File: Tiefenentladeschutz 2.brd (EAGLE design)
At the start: 60 x 60 mm, 23 parts, among them IC1 ICL7665CSA, Q1 NMOSFET-D2PAK-7

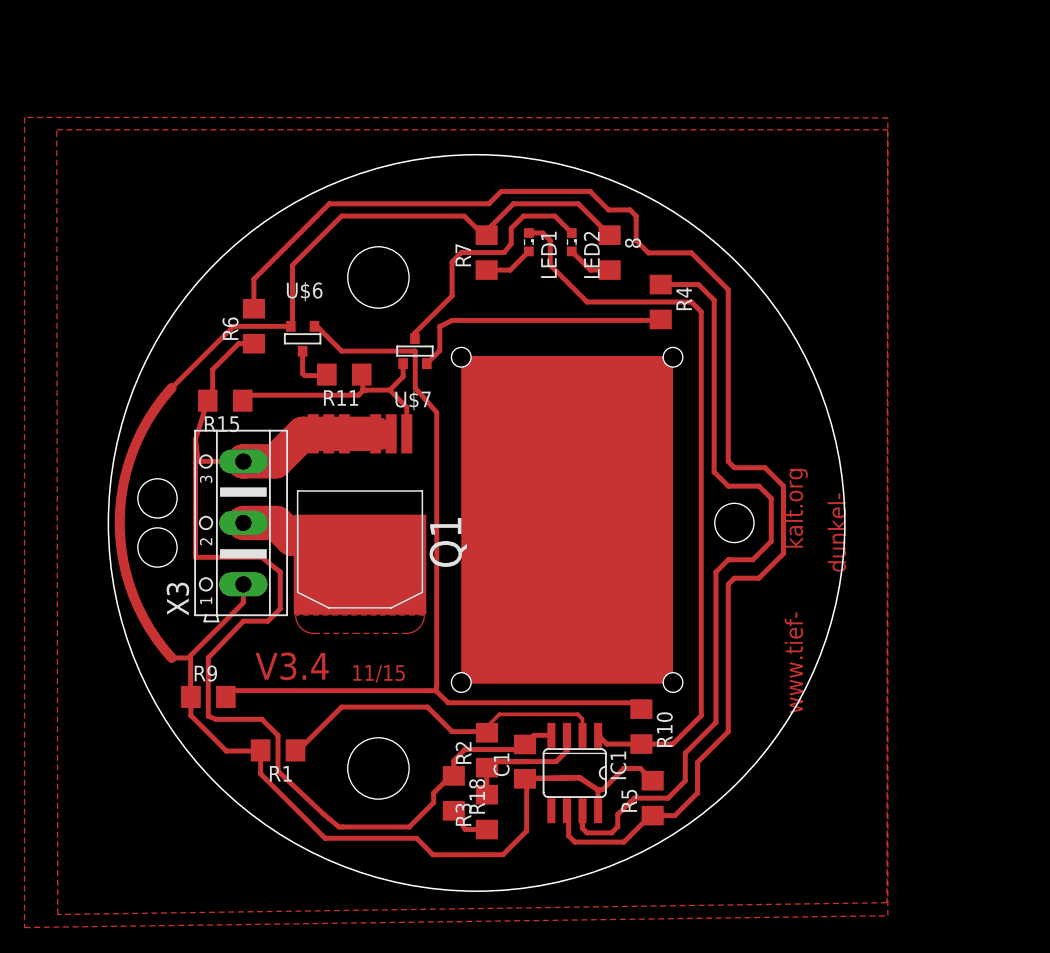
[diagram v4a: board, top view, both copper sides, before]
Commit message: 3.5
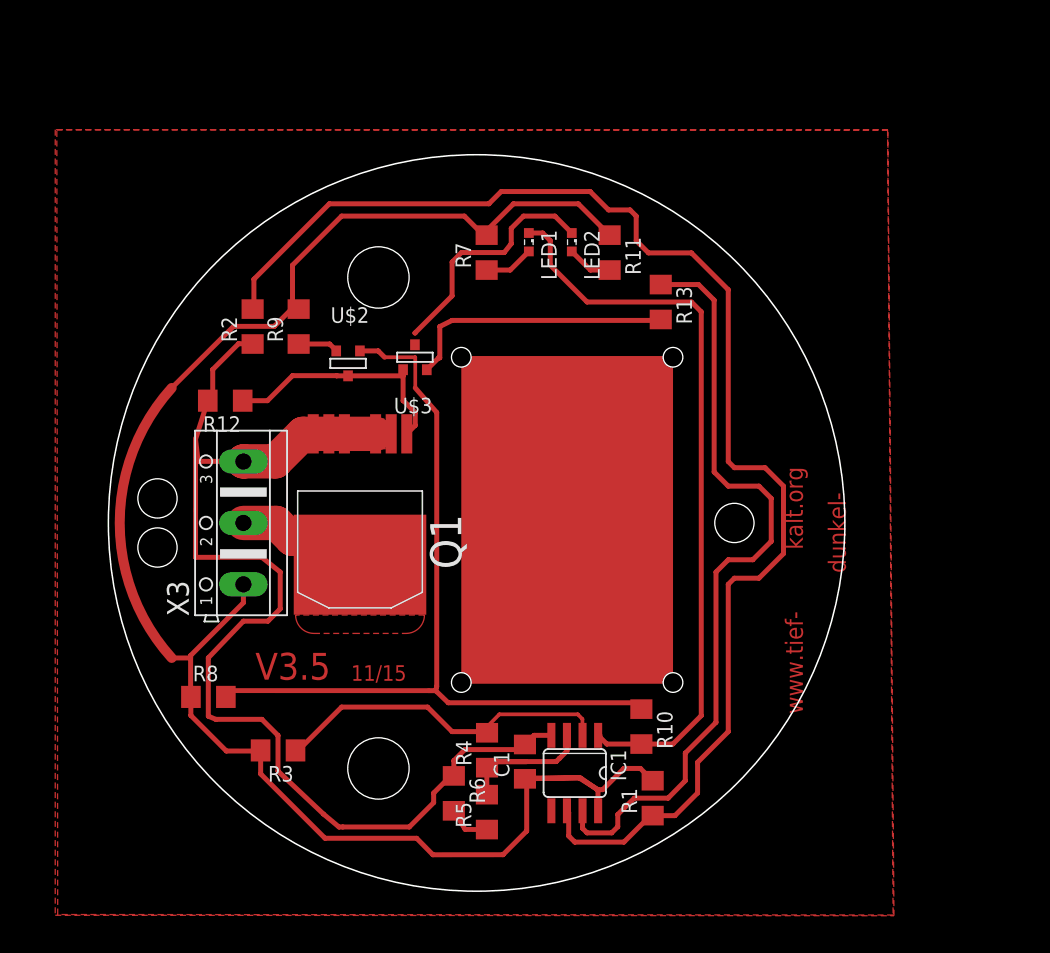
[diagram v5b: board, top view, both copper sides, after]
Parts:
- removed 8, R18: 5,6k, eagle-ltspice:R1206
- removed U$6: IRLML9301, 0liver:SOT-23
- removed U$7: IRLML6346, 0liver:SOT-23
- added R13: 0, eagle-ltspice:R1206
- added R8: 470k, eagle-ltspice:R1206
- added U$2: IRLML9301, 0liver:SOT-23
- added U$3: IRLML6346, 0liver:SOT-23
- R1: value 100k -> 820k
- R11: value 68k -> 5,6k
- R12: value 470k -> 100k
- R2: value 750k -> 100k
- R3: value 120k -> 100k
- R4: value 0 -> 750k
- R5: value 820k -> 120k
- R6: value 100k -> 5,6k
- R9: value 470k -> 68k
- moved R6 41.4 mm to (28.1, 7.97), turned to 270 degrees
- moved R2 39.4 mm to (11.8, 46.0)
- moved R4 39.2 mm to (30.8, 11.5), turned to 90 degrees
- moved R9 31.1 mm to (15.5, 46.0), turned to 90 degrees
- moved R1 30.8 mm to (44.3, 7.58), turned to 90 degrees
- moved R11 23.8 mm to (40.8, 52.0), turned to 270 degrees
- moved R3 17.7 mm to (13.8, 11.5), turned to 180 degrees
- moved R5 13.6 mm to (30.8, 6.44)
- renumbered R15 to R12
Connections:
- removed net N$10: R11.2, U$6.1
- new net N$8: R9.1, U$2.2
- net GND: now also R2.1; no longer R18.1
- net N$11: now also U$3.1; no longer U$7.1
- net N$13: now also R3.1, R4.2; no longer R1.1, R2.2
- net N$2: now also R4.1, R5.2; no longer R2.1, R3.2
- net N$22: now also U$2.1, U$3.3; no longer R11.1, U$7.3
- net N$23: now also R13.1; no longer R4.1
- net N$26: now also R5.1, R6.2; no longer R18.2, R3.1
- net N$3: now also R13.2, U$3.2; no longer R4.2, U$7.2
- net N$4: now also R1.1, R2.2; no longer R5.1, R6.2
- net N$5: now also R11.2; no longer 8.2
- net N$7: now also R8.2, U$2.3; no longer R9.2, U$6.3
- net V+: now also R11.1, R3.2, R8.1, R9.2; no longer 8.1, R5.2, R9.1, U$6.2
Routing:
- net N$7: track 72.5 -> 67.7 mm
- net N$10: track 4.10 -> 0.00 mm
- net N$8: track 0.00 -> 3.31 mm
- net N$22: track 20.7 -> 19.9 mm
- net N$3: track 21.8 -> 22.3 mm
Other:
- board text added: "V3.5"
- board text removed: "V3.4"

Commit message: 3.7
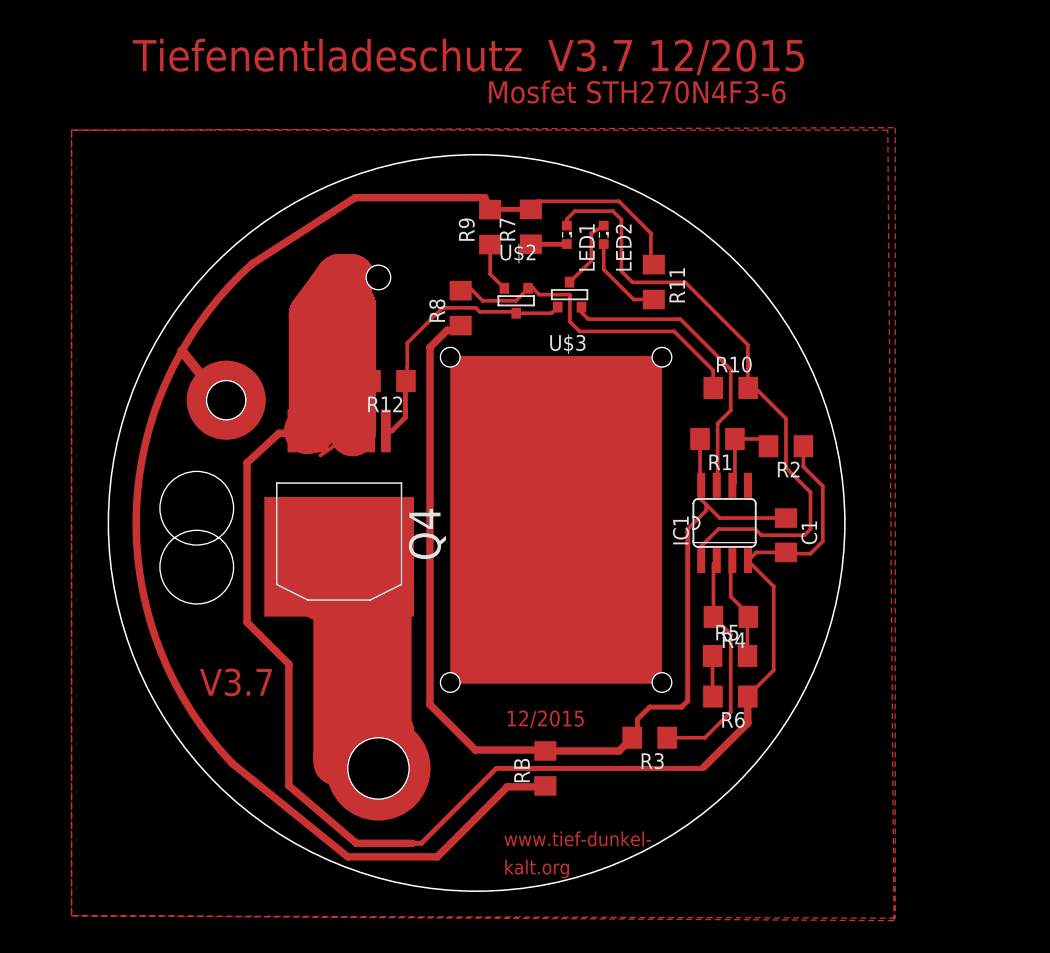
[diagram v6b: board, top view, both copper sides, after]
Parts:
- removed Q1: NMOSFET-D2PAK-7, D2pak-7:D2PAK-7
- removed R13: 0, eagle-ltspice:R1206
- removed X3: (no value), con-ptr500:AK500/3
- added Q4: NMOSFET-D2PAK-7, D2pak-7:H2PAK-6
- added RB: 0, eagle-ltspice:R1206
- added U$4: (no value), 0liver:PIN
- added U$6, U$7: (no value), 0liver:PIN-1.27
- moved R2 44.5 mm to (55.2, 36.2), turned to 180 degrees
- moved R8 37.8 mm to (28.7, 47.5), turned to 90 degrees
- moved R3 30.3 mm to (44.1, 12.5)
- moved R1 29.7 mm to (49.6, 36.8), turned to 180 degrees
- moved R10 28.5 mm to (50.7, 41.0), turned to 0 degrees
- moved C1 28.1 mm to (55.2, 29.0), turned to 270 degrees
- moved R6 23.9 mm to (50.7, 15.9), turned to 180 degrees
- moved IC1 23.8 mm to (50.2, 30.0), turned to 0 degrees
- moved R5 23.5 mm to (50.6, 19.2), turned to 0 degrees
- moved R4 22.6 mm to (50.7, 22.3), turned to 180 degrees
- moved R9 17.6 mm to (31.1, 54.1)
- moved U$2 14.6 mm to (33.2, 48.1)
- moved U$3 13.6 mm to (37.6, 48.6)
- moved R12 13.4 mm to (22.8, 41.6)
- moved R11 4.33 mm to (44.4, 49.6)
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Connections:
- removed net N$23: IC1.7, R13.1
- new net N$10: R9.2, RB.1
- net GND: now also Q4.S1, Q4.S2, Q4.S3, Q4.S4, Q4.S5, U$6.P$1; no longer Q1.S1, Q1.S2, Q1.S3, Q1.S4, Q1.S5, X3.3
- net N$1: now also Q4.D, U$7.P$1; no longer Q1.D, X3.2
- net N$22: now also Q4.G; no longer Q1.G
- net N$3: now also IC1.7; no longer R13.2
- net V+: now also RB.2, U$4.P$1; no longer R9.2, X3.1
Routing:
- net N$4: track 111.4 -> 6.83 mm
- net N$10: track 0.00 -> 94.5 mm
- net N$23: track 63.8 -> 0.00 mm
- net N$1: track 10.9 -> 62.0 mm
- net GND: track 104.2 -> 153.9 mm
- net N$7: track 67.7 -> 26.9 mm
- net V+: track 142.0 -> 115.7 mm
- net N$11: track 19.7 -> 5.91 mm
- net N$16: track 60.6 -> 51.0 mm
- net N$13: track 28.1 -> 19.1 mm
- net N$2: track 15.0 -> 8.45 mm
- net N$5: track 3.71 -> 7.17 mm
- net N$22: track 19.9 -> 22.0 mm
- net N$3: track 22.3 -> 24.4 mm
- net N$6: track 4.07 -> 2.95 mm
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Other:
- board text added: "12/2015"
- board text added: "Mosfet STH270N4F3-6"
- board text added: "Tiefenentladeschutz V3.7 12/2015"
- board text added: "V3.7"
- board text added: "www.tief-dunkel- kalt.org"
- board text removed: "V3.5"
- board text removed: "dunkel-"
- board text removed: "www.tief- kalt.org"
